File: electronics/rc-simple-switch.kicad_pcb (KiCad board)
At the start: 2 copper layers, 22 x 8 mm, 13 parts, among them K1 CONN_3, K2 CONN_3, P1 CONN_1, P2 CONN_1, P3 CONN_1, P4 CONN_1, P5 CONN_1, Q1 PMV30UN, U1 PIC10F200

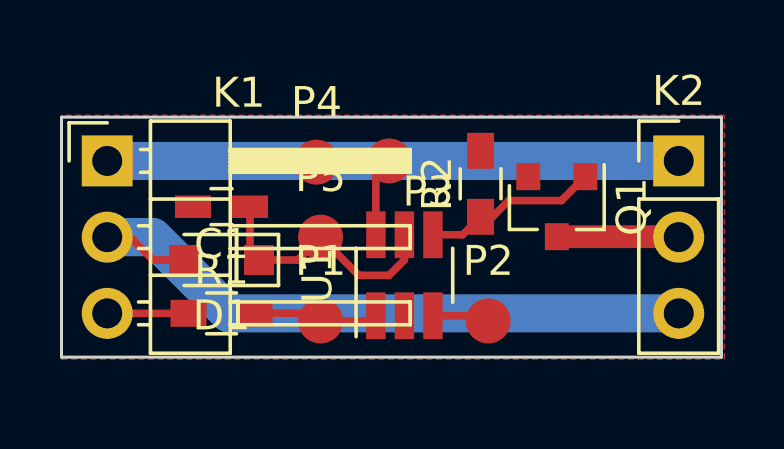
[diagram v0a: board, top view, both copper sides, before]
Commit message: Finish PCB re-layout
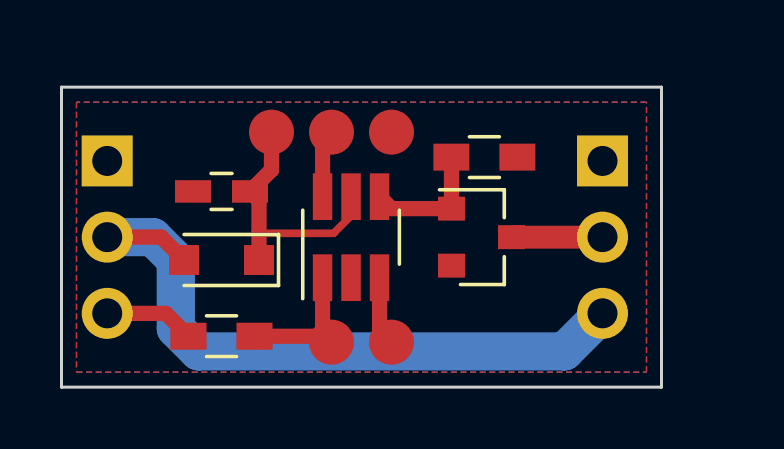
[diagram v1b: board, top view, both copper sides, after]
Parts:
- K1, K2: moved to B.Cu
- R1: value 680 -> 1k
- moved P5 3.86 mm to (107.0, 96.5)
- moved P2 3.30 mm to (111.0, 103.5)
- moved Q1 2.71 mm to (114.0, 100.0), turned to 0 degrees
- moved P4 2.69 mm to (111.0, 96.5)
- moved K2 2.54 mm to (118.0, 97.5), turned to 180 degrees
- moved U1 2.18 mm to (109.7, 100.0)
- moved P3 2.15 mm to (109.0, 96.5)
- moved R2 0.90 mm to (114.1, 97.3), turned to 0 degrees
- moved P1 0.79 mm to (109.0, 103.5)
- moved R1 0.76 mm to (105.3, 103.3)
- moved C1 0.51 mm to (105.3, 98.5)
- turned K1 to 180 degrees
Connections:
- net Net-(K1-Pad3) renamed /S
- net Net-(K2-Pad2) renamed /SW
- net Net-(P1-Pad1) renamed /DAT
- net Net-(P2-Pad1) renamed /CLK
- net Net-(P3-Pad1) renamed /VPP
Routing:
- net GND: track 19.0 -> 0.00 mm
- net /OUT: track 6.18 -> 4.28 mm
- net /SW: track 4.07 -> 3.03 mm
- net /DAT: track 4.22 -> 5.20 mm
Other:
- board size 22 x 8 mm -> 20 x 10 mm
- board text added: "+"
- board text added: "-"
- board text added: "LANE Boys RC"
- board text added: "RC switch"
- board text added: "S"
- board text added: "SW"
